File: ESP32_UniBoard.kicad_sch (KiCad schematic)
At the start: 31 parts, among them J1 USB_C_Receptacle_USB2.0, J2 Conn_01x06_Socket, J3 Hirose DF40C, SW1 SW_Push, SW2 SW_Push, U1 ESP32-S3-WROOM-1, U2 SPX3819M5-L-3-3, U3 USBLC6-2SC6

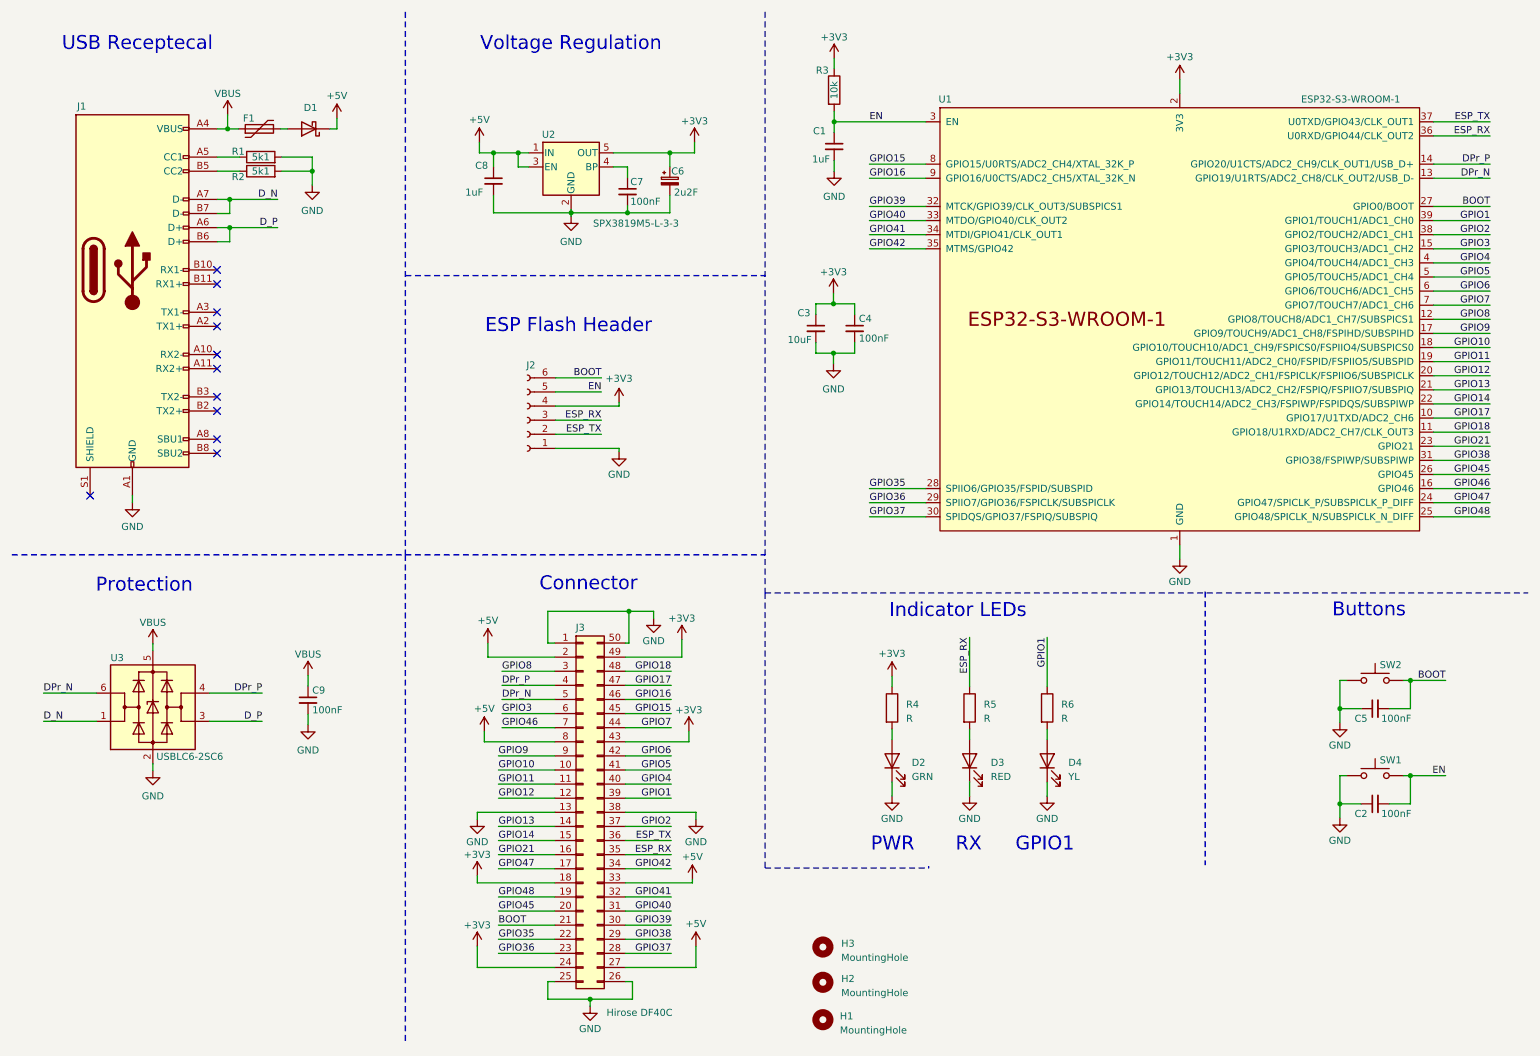
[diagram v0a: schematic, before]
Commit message: Adjustments in Schematic and PCB
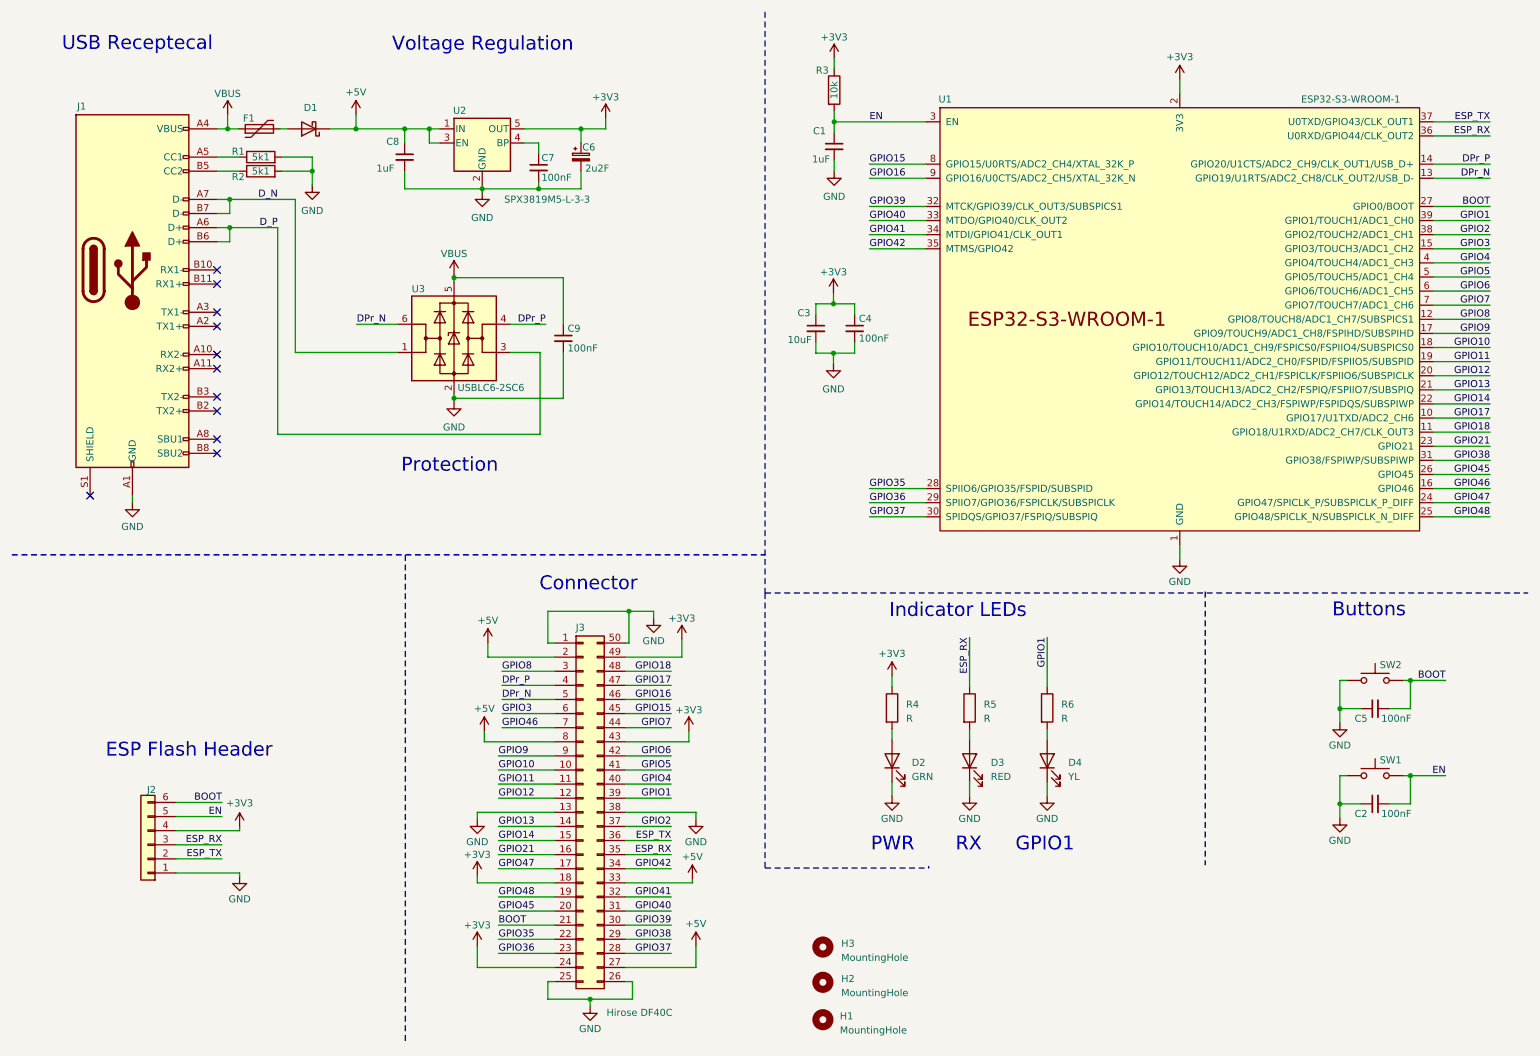
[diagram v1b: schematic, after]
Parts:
- J2: symbol Connector:Conn_01x06_Socket -> Connector_Generic:Conn_01x06
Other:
- moved on the sheet: C6, C7, C8, C9, U2, U3

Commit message: -
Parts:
- J3: footprint Hirose_Connector_DF40C:Hirose_DF40C-50 -> Hirose_Connector_DF40C:Hirose_DF40C-50DS
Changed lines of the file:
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@@
       (effects (font (size 1.27 1.27)))
     )
-    (property "Footprint" "Hirose_Connector_DF40C:Hirose_DF40C-50" (at 114.808 156.083 0)
+    (property "Footprint" "Hirose_Connector_DF40C:Hirose_DF40C-50DS" (at 114.808 156.083 0)
       (effects (font (size 1.27 1.27)) hide)
     )
